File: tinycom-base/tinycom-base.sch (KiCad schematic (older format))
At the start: 36 parts, among them J1 MICRO_SD_HINGE, P1 CONN_02X10, P2 CONN_02X10, P3 USB_A, P4 USB_OTG, U1 SY8008BAAC, U2 AXP209, U3 SY8008BAAC, U4 RTL8188, U5 rainsun-antenna

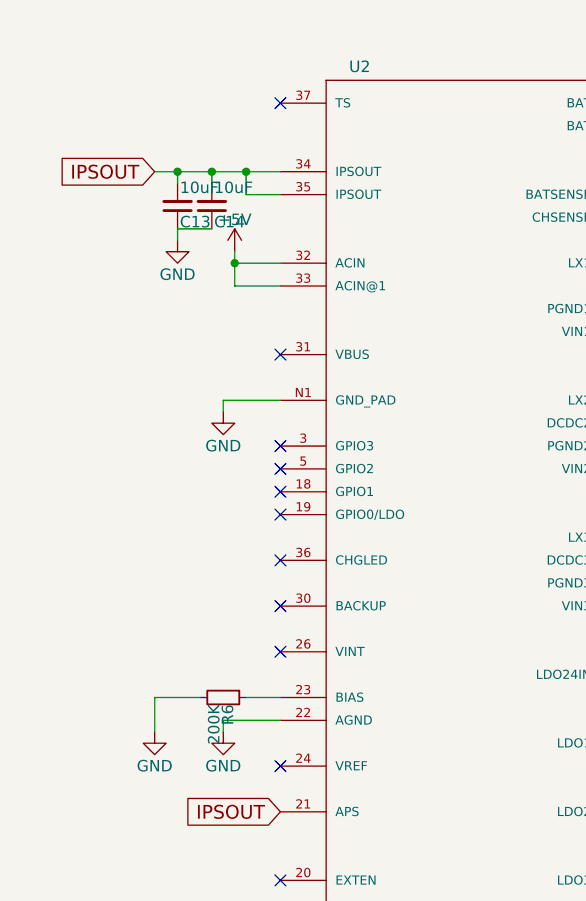
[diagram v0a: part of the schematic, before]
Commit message: route
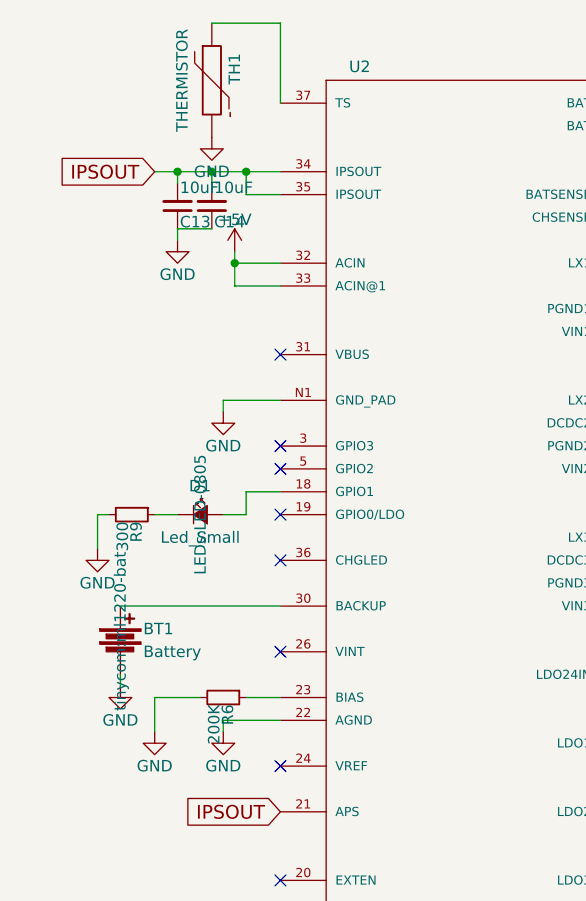
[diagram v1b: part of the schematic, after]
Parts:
- added BT1: Battery, tinycom:ml1220-bat, symbol Battery
- added D1: Led_Small, LEDs:LED-0805, symbol Led_Small
- added R9: 300, Resistors_SMD:R_0805, symbol R_Small
- added TH1: THERMISTOR, Discret:R1, symbol THERMISTOR
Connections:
- net GND: now also BT1.2, R9.2, TH1.2
- net at U2.18 (GPIO1): now also D1.2 (A)
- net at U2.30 (BACKUP): now also BT1.1
- net at U2.37 (TS): now also TH1.1
- new net: D1.1 (K), R9.1
- no-connect marks 23 -> 20
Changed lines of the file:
@@
 $EndComp
 $Comp
-L +5V #PWR16
+L +5V #PWR19
 U 1 1 562DA8F7
 P 5250 4200
-F 0 "#PWR16" H 5250 4050 50  0001 C CNN
+F 0 "#PWR19" H 5250 4050 50  0001 C CNN
 F 1 "+5V" H 5250 4340 50  0000 C CNN
 F 2 "" H 5250 4200 60  0000 C CNN
@@
 $EndComp
 $Comp
-L GND #PWR17
+L GND #PWR20
 U 1 1 562DA928
 P 5250 4600
-F 0 "#PWR17" H 5250 4350 50  0001 C CNN
+F 0 "#PWR20" H 5250 4350 50  0001 C CNN
 F 1 "GND" H 5250 4450 50  0000 C CNN
 F 2 "" H 5250 4600 60  0000 C CNN
@@
 $EndComp
 $Comp
-L +5V #PWR18
+L +5V #PWR21
 U 1 1 562DAC42
 P 5300 5050
-F 0 "#PWR18" H 5300 4900 50  0001 C CNN
+F 0 "#PWR21" H 5300 4900 50  0001 C CNN
 F 1 "+5V" H 5300 5190 50  0000 C CNN
 F 2 "" H 5300 5050 60  0000 C CNN
@@
 $EndComp
 $Comp
-L GND #PWR19
+L GND #PWR22
 U 1 1 562DAC77
 P 5300 5500
-F 0 "#PWR19" H 5300 5250 50  0001 C CNN
+F 0 "#PWR22" H 5300 5250 50  0001 C CNN
 F 1 "GND" H 5300 5350 50  0000 C CNN
 F 2 "" H 5300 5500 60  0000 C CNN
@@
 UD0_P
 $Comp
-L GND #PWR22
+L GND #PWR25
 U 1 1 562DAF0B
 P 6050 1300
-F 0 "#PWR22" H 6050 1050 50  0001 C CNN
+F 0 "#PWR25" H 6050 1050 50  0001 C CNN
 F 1 "GND" H 6050 1150 50  0000 C CNN
 F 2 "" H 6050 1300 60  0000 C CNN
@@
 $EndComp
 $Comp
-L +5V #PWR20
+L +5V #PWR23
 U 1 1 562DAF87
 P 5950 900
-F 0 "#PWR20" H 5950 750 50  0001 C CNN
+F 0 "#PWR23" H 5950 750 50  0001 C CNN
 F 1 "+5V" H 5950 1040 50  0000 C CNN
 F 2 "" H 5950 900 60  0000 C CNN
@@
 $EndComp
 $Comp
-L +5V #PWR23
+L +5V #PWR26
 U 1 1 562DB2B7
 P 6400 1950
-F 0 "#PWR23" H 6400 1800 50  0001 C CNN
+F 0 "#PWR26" H 6400 1800 50  0001 C CNN
 F 1 "+5V" H 6400 2090 50  0000 C CNN
 F 2 "" H 6400 1950 60  0000 C CNN
@@
 $EndComp
 $Comp
-L GND #PWR24
+L GND #PWR27
 U 1 1 562DB346
 P 6550 2300
-F 0 "#PWR24" H 6550 2050 50  0001 C CNN
+F 0 "#PWR27" H 6550 2050 50  0001 C CNN
 F 1 "GND" H 6550 2150 50  0000 C CNN
 F 2 "" H 6550 2300 60  0000 C CNN
@@
 UD0_N
 $Comp
-L GND #PWR15
+L GND #PWR18
 U 1 1 562DAEC4
 P 5050 6000
-F 0 "#PWR15" H 5050 5750 50  0001 C CNN
+F 0 "#PWR18" H 5050 5750 50  0001 C CNN
 F 1 "GND" H 5050 5850 50  0000 C CNN
 F 2 "" H 5050 6000 60  0000 C CNN
@@
 $EndComp
 $Comp
-L GND #PWR21
+L GND #PWR24
 U 1 1 562DA997
 P 6000 7200
-F 0 "#PWR21" H 6000 6950 50  0001 C CNN
+F 0 "#PWR24" H 6000 6950 50  0001 C CNN
 F 1 "GND" H 6000 7050 50  0000 C CNN
 F 2 "" H 6000 7200 60  0000 C CNN
@@
 SDC0_D1
 $Comp
-L GND #PWR28
+L GND #PWR31
 U 1 1 562DAEE9
 P 7450 4950
-F 0 "#PWR28" H 7450 4700 50  0001 C CNN
+F 0 "#PWR31" H 7450 4700 50  0001 C CNN
 F 1 "GND" H 7450 4800 50  0000 C CNN
 F 2 "" H 7450 4950 60  0000 C CNN
@@
 $EndComp
 $Comp
-L GND #PWR32
+L GND #PWR35
 U 1 1 562DAF47
 P 9050 5450
-F 0 "#PWR32" H 9050 5200 50  0001 C CNN
+F 0 "#PWR35" H 9050 5200 50  0001 C CNN
 F 1 "GND" H 9050 5300 50  0000 C CNN
 F 2 "" H 9050 5450 60  0000 C CNN
@@
 $EndComp
 $Comp
-L +3.3V #PWR26
+L +3.3V #PWR29
 U 1 1 562DB369
 P 7300 4000
-F 0 "#PWR26" H 7300 3850 50  0001 C CNN
+F 0 "#PWR29" H 7300 3850 50  0001 C CNN
 F 1 "+3.3V" H 7300 4140 50  0000 C CNN
 F 2 "" H 7300 4000 60  0000 C CNN
@@
 $EndComp
 $Comp
-L GND #PWR29
+L GND #PWR32
 U 1 1 562DB89F
 P 7950 1550
-F 0 "#PWR29" H 7950 1300 50  0001 C CNN
+F 0 "#PWR32" H 7950 1300 50  0001 C CNN
 F 1 "GND" H 7950 1400 50  0000 C CNN
 F 2 "" H 7950 1550 60  0000 C CNN
@@
 $EndComp
 $Comp
-L +3.3V #PWR30
+L +3.3V #PWR33
 U 1 1 562DBC47
 P 8300 900
-F 0 "#PWR30" H 8300 750 50  0001 C CNN
+F 0 "#PWR33" H 8300 750 50  0001 C CNN
 F 1 "+3.3V" H 8300 1040 50  0000 C CNN
 F 2 "" H 8300 900 60  0000 C CNN
@@
 $EndComp
 $Comp
-L GND #PWR31
+L GND #PWR34
 U 1 1 562F9FD4
 P 8350 2700
-F 0 "#PWR31" H 8350 2450 50  0001 C CNN
+F 0 "#PWR34" H 8350 2450 50  0001 C CNN
 F 1 "GND" H 8350 2550 50  0000 C CNN
 F 2 "" H 8350 2700 60  0000 C CNN
@@
 $EndComp
 $Comp
-L GND #PWR13
+L GND #PWR16
 U 1 1 5634B03F
 P 4900 4550
-F 0 "#PWR13" H 4900 4300 50  0001 C CNN
+F 0 "#PWR16" H 4900 4300 50  0001 C CNN
 F 1 "GND" H 4900 4400 50  0000 C CNN
 F 2 "" H 4900 4550 60  0000 C CNN
@@
 $EndComp
 $Comp
-L GND #PWR14
+L GND #PWR17
 U 1 1 5634B0B0
 P 4900 5400
-F 0 "#PWR14" H 4900 5150 50  0001 C CNN
+F 0 "#PWR17" H 4900 5150 50  0001 C CNN
 F 1 "GND" H 4900 5250 50  0000 C CNN
 F 2 "" H 4900 5400 60  0000 C CNN
@@
 $EndComp
 $Comp
-L GND #PWR25
+L GND #PWR28
 U 1 1 565A1DA6
 P 7100 5650
-F 0 "#PWR25" H 7100 5400 50  0001 C CNN
+F 0 "#PWR28" H 7100 5400 50  0001 C CNN
 F 1 "GND" H 7100 5500 50  0000 C CNN
 F 2 "" H 7100 5650 60  0000 C CNN
@@
 $EndComp
 $Comp
-L GND #PWR11
+L GND #PWR14
 U 1 1 567CDE13
 P 3600 2600
-F 0 "#PWR11" H 3600 2350 50  0001 C CNN
+F 0 "#PWR14" H 3600 2350 50  0001 C CNN
 F 1 "GND" H 3600 2450 50  0000 C CNN
 F 2 "" H 3600 2600 50  0000 C CNN
@@
 VCC_12_INT
 $Comp
-L GND #PWR12
+L GND #PWR15
 U 1 1 567CF2F6
 P 3650 3200
-F 0 "#PWR12" H 3650 2950 50  0001 C CNN
+F 0 "#PWR15" H 3650 2950 50  0001 C CNN
 F 1 "GND" H 3650 3050 50  0000 C CNN
 F 2 "" H 3650 3200 50  0000 C CNN
@@
 $EndComp
 $Comp
-L GND #PWR2
+L GND #PWR4
 U 1 1 567D1B80
 P 850 5300
-F 0 "#PWR2" H 850 5050 50  0001 C CNN
+F 0 "#PWR4" H 850 5050 50  0001 C CNN
 F 1 "GND" H 850 5150 50  0000 C CNN
 F 2 "" H 850 5300 50  0000 C CNN
@@
 $EndComp
 $Comp
-L +5V #PWR6
+L +5V #PWR9
 U 1 1 567D3261
 P 1200 1700
-F 0 "#PWR6" H 1200 1550 50  0001 C CNN
+F 0 "#PWR9" H 1200 1550 50  0001 C CNN
 F 1 "+5V" H 1200 1840 50  0000 C CNN
 F 2 "" H 1200 1700 60  0000 C CNN
@@
 $EndComp
 $Comp
-L GND #PWR7
+L GND #PWR10
 U 1 1 567D3BC0
 P 3250 6000
-F 0 "#PWR7" H 3250 5750 50  0001 C CNN
+F 0 "#PWR10" H 3250 5750 50  0001 C CNN
 F 1 "GND" H 3250 5850 50  0000 C CNN
 F 2 "" H 3250 6000 50  0000 C CNN
@@
 $EndComp
 $Comp
-L GND #PWR9
+L GND #PWR12
 U 1 1 567D4184
 P 3500 3900
-F 0 "#PWR9" H 3500 3650 50  0001 C CNN
+F 0 "#PWR12" H 3500 3650 50  0001 C CNN
 F 1 "GND" H 3500 3750 50  0000 C CNN
 F 2 "" H 3500 3900 50  0000 C CNN
@@
 $EndComp
 $Comp
-L GND #PWR10
+L GND #PWR13
 U 1 1 567D4986
 P 3500 4400
-F 0 "#PWR10" H 3500 4150 50  0001 C CNN
+F 0 "#PWR13" H 3500 4150 50  0001 C CNN
 F 1 "GND" H 3500 4250 50  0000 C CNN
 F 2 "" H 3500 4400 50  0000 C CNN
@@
 IPSOUT
 $Comp
-L GND #PWR5
+L GND #PWR8
 U 1 1 567D57C2
 P 1150 3800
-F 0 "#PWR5" H 1150 3550 50  0001 C CNN
+F 0 "#PWR8" H 1150 3550 50  0001 C CNN
 F 1 "GND" H 1150 3650 50  0000 C CNN
 F 2 "" H 1150 3800 50  0000 C CNN
@@
 $EndComp
 $Comp
-L GND #PWR4
+L GND #PWR7
 U 1 1 567D5BDE
 P 1150 2400
-F 0 "#PWR4" H 1150 2150 50  0001 C CNN
+F 0 "#PWR7" H 1150 2150 50  0001 C CNN
 F 1 "GND" H 1150 2250 50  0000 C CNN
 F 2 "" H 1150 2400 50  0000 C CNN
@@
 NoConn ~ 3000 4450
 $Comp
-L GND #PWR8
+L GND #PWR11
 U 1 1 567D6614
 P 3500 2000
-F 0 "#PWR8" H 3500 1750 50  0001 C CNN
+F 0 "#PWR11" H 3500 1750 50  0001 C CNN
 F 1 "GND" H 3500 1850 50  0000 C CNN
 F 2 "" H 3500 2000 50  0000 C CNN
@@
 NoConn ~ 1400 2550
 NoConn ~ 1400 2650
-NoConn ~ 1400 2750
 NoConn ~ 1400 2850
 $Comp
@@
 $EndComp
 $Comp
-L GND #PWR27
+L GND #PWR30
 U 1 1 567D811C
 P 7400 6300
-F 0 "#PWR27" H 7400 6050 50  0001 C CNN
+F 0 "#PWR30" H 7400 6050 50  0001 C CNN
 F 1 "GND" H 7400 6150 50  0000 C CNN
 F 2 "" H 7400 6300 50  0000 C CNN
@@
 	1    0    0    -1
 $EndComp
-NoConn ~ 1400 1050
 NoConn ~ 3000 1750
 NoConn ~ 3000 2050
 NoConn ~ 1400 2150
 NoConn ~ 1400 3050
-NoConn ~ 1400 3250
 Text GLabel 1400 5450 0    60   Input ~ 0
 IPSOUT
@@
 $EndComp
 $Comp
-L GND #PWR1
+L GND #PWR3
 U 1 1 567E433F
 P 850 3800
-F 0 "#PWR1" H 850 3550 50  0001 C CNN
+F 0 "#PWR3" H 850 3550 50  0001 C CNN
 F 1 "GND" H 850 3650 50  0000 C CNN
 F 2 "" H 850 3800 50  0000 C CNN
@@
 $EndComp
 $Comp
-L GND #PWR3
+L GND #PWR5
 U 1 1 568508CF
 P 950 1650
-F 0 "#PWR3" H 950 1400 50  0001 C CNN
+F 0 "#PWR5" H 950 1400 50  0001 C CNN
 F 1 "GND" H 950 1500 50  0000 C CNN
 F 2 "" H 950 1650 50  0000 C CNN
@@
 Wire Wire Line
 	1100 1600 950  1600
+$Comp
+L THERMISTOR TH1
+U 1 1 56864773
+P 1100 950
+F 0 "TH1" V 1200 1000 50  0000 C CNN
+F 1 "THERMISTOR" V 1000 950 50  0000 C BNN
+F 2 "Discret:R1" H 1100 950 50  0001 C CNN
+F 3 "" H 1100 950 50  0000 C CNN
+	1    1100 950
+	1    0    0    -1
+$EndComp
+Wire Wire Line
+	1400 1050 1400 700
+Wire Wire Line
+	1400 700  1100 700
+$Comp
+L GND #PWR6
+U 1 1 56864E38
+P 1100 1200
+F 0 "#PWR6" H 1100 950 50  0001 C CNN
+F 1 "GND" H 1100 1050 50  0000 C CNN
+F 2 "" H 1100 1200 50  0000 C CNN
+F 3 "" H 1100 1200 50  0000 C CNN
+	1    1100 1200
+	1    0    0    -1
+$EndComp
+$Comp
+L Led_Small D1
+U 1 1 56865F44
+P 1050 2850
+F 0 "D1" H 1000 2975 50  0000 L CNN
+F 1 "Led_Small" H 875 2750 50  0000 L CNN
+F 2 "LEDs:LED-0805" V 1050 2850 50  0000 C CNN
+F 3 "" V 1050 2850 50  0000 C CNN
+	1    1050 2850
+	1    0    0    -1
+$EndComp
+$Comp
+L R_Small R9
+U 1 1 568663CD
+P 750 2850
+F 0 "R9" H 780 2870 50  0000 L CNN
+F 1 "300" H 780 2810 50  0000 L CNN
+F 2 "Resistors_SMD:R_0805" H 750 2850 60  0001 C CNN
+F 3 "" H 750 2850 60  0000 C CNN
+	1    750  2850
+	0    1    1    0
+$EndComp
+Wire Wire Line
+	950  2850 850  2850
+$Comp
+L GND #PWR1
+U 1 1 56866572
+P 600 3000
+F 0 "#PWR1" H 600 2750 50  0001 C CNN
+F 1 "GND" H 600 2850 50  0000 C CNN
+F 2 "" H 600 3000 50  0000 C CNN
+F 3 "" H 600 3000 50  0000 C CNN
+	1    600  3000
+	1    0    0    -1
+$EndComp
+Wire Wire Line
+	650  2850 600  2850
+Wire Wire Line
+	600  2850 600  3000
+Wire Wire Line
+	1150 2850 1250 2850
+Wire Wire Line
+	1250 2850 1250 2750
+Wire Wire Line
+	1250 2750 1400 2750
+$Comp
+L Battery BT1
+U 1 1 5686793B
+P 700 3400
+F 0 "BT1" H 800 3450 50  0000 L CNN
+F 1 "Battery" H 800 3350 50  0000 L CNN
+F 2 "tinycom:ml1220-bat" V 700 3440 50  0000 C CNN
+F 3 "" V 700 3440 50  0000 C CNN
+	1    700  3400
+	1    0    0    -1
+$EndComp
+Wire Wire Line
+	700  3250 1400 3250
+$Comp
+L GND #PWR2
+U 1 1 568683F8
+P 700 3600
+F 0 "#PWR2" H 700 3350 50  0001 C CNN
+F 1 "GND" H 700 3450 50  0000 C CNN
+F 2 "" H 700 3600 50  0000 C CNN
+F 3 "" H 700 3600 50  0000 C CNN
+	1    700  3600
+	1    0    0    -1
+$EndComp
+Wire Wire Line
+	700  3550 700  3600
 $EndSCHEMATC
